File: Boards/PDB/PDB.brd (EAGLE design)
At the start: 160 x 101.6 mm, 49 parts, among them Q1 NMOS, Q2 IRFML8244, Q3 PMOS, Q4 PMOS, Q5 PMOS

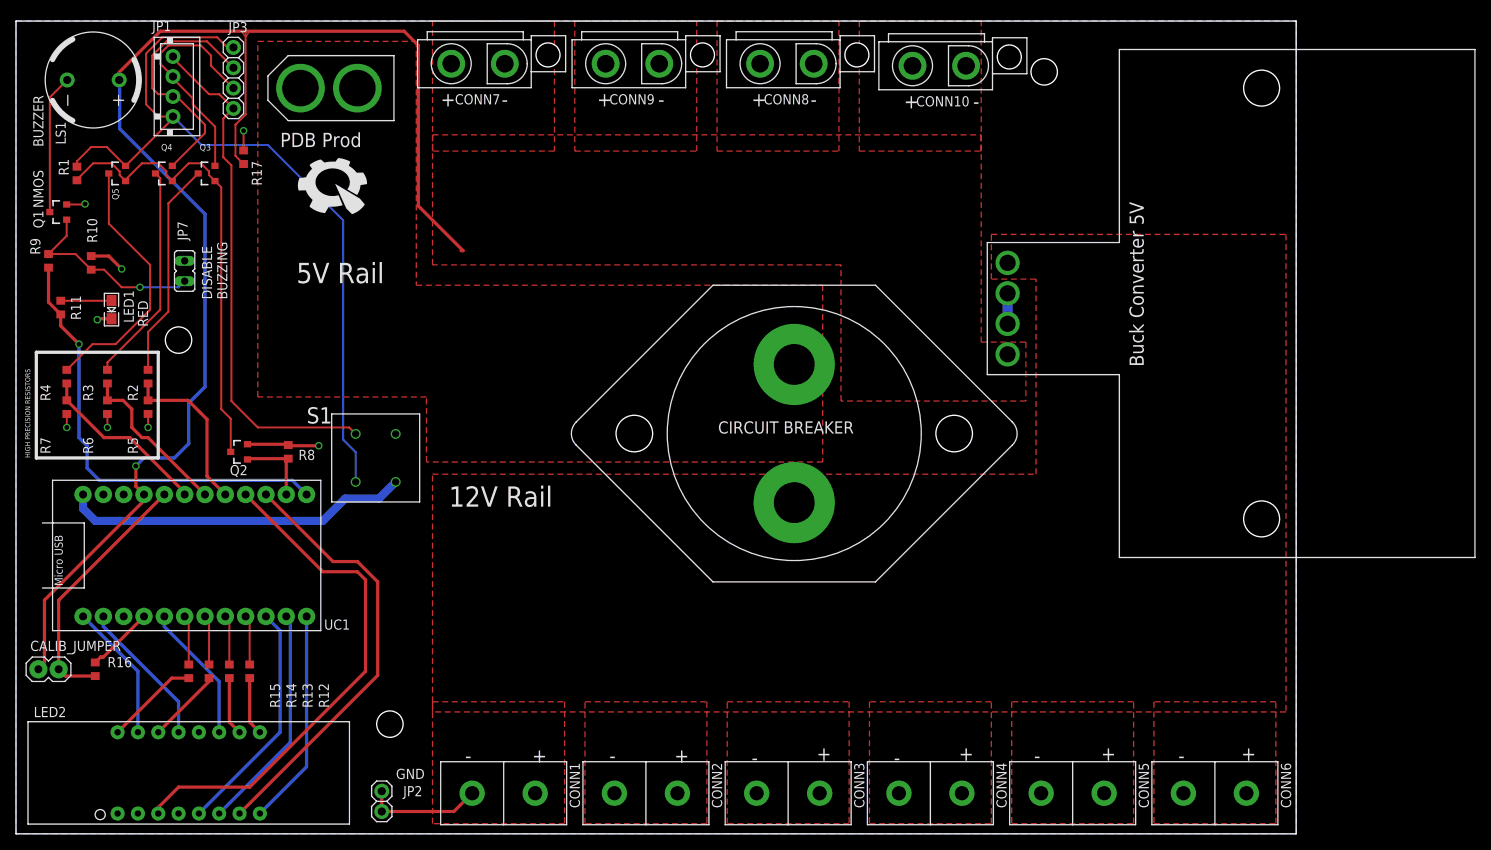
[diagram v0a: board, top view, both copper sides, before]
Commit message: REV B PLEASE WORK
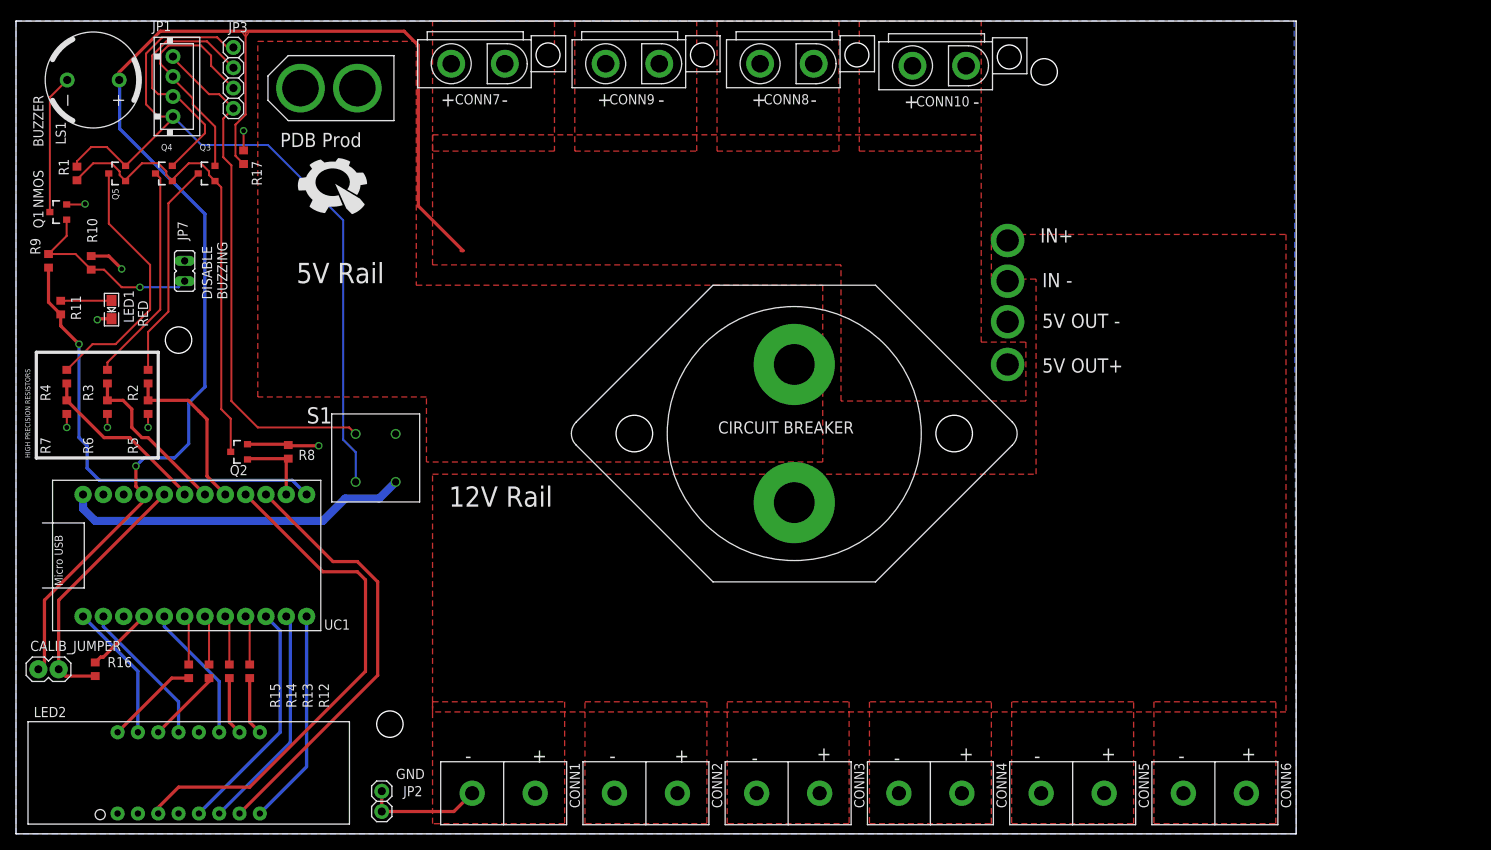
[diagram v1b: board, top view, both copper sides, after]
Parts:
- removed U$7: BUCK_CONVERTER_5V, pie:BUCK_CONVERTER_5V
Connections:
- net 12V: no longer U$7.IN+
- net 5V: no longer U$7.OUT+
- net GND: no longer U$7.IN-, U$7.OUT-
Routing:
- net GND: track 52.3 -> 48.5 mm, vias 8 -> 10
- net 5V: vias 1 -> 2
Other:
- board text added: "5V OUT -"
- board text added: "5V OUT+"
- board text added: "IN -"
- board text added: "IN+"
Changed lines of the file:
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@@
 <text x="80.264" y="90.932" size="1.778" layer="21">-</text>
 <text x="60.706" y="90.932" size="1.778" layer="21">-</text>
+<text x="128.016" y="73.914" size="1.778" layer="21">IN+</text>
+<text x="128.27" y="68.326" size="1.778" layer="21" font="vector">IN -</text>
+<text x="128.27" y="63.246" size="1.778" layer="21">5V OUT -</text>
+<text x="128.27" y="57.658" size="1.778" layer="21">5V OUT+</text>
 </plain>
 <attributes>
@@
 <element name="U$5" library="pie" package="STAND-OFF" value="" x="20.32" y="61.722"/>
 <element name="U$6" library="pie" package="PIE-LOGO-SMALL" value="" x="39.878" y="81.28"/>
-<element name="U$7" library="pie" package="BUCK_CONVERTER_5V" value="BUCK_CONVERTER_5V" x="155.702" y="66.294" smashed="yes" rot="R90"/>
 <element name="JP1" library="pie" package="XH_CONNECTOR_4POS_2.5MM" value="XH_CONN" x="19.812" y="93.218" smashed="yes" rot="R270">
 <attribute name="PIE-INT-REF-NUM" value="XH-4POS" x="71.882" y="104.648" size="1.778" layer="27" rot="R270" display="off"/>
@@
 <polygon width="1.1938" layer="16" rank="6">
 <vertex x="0" y="101.6"/>
-<vertex x="160.02" y="101.6"/>
+<vertex x="159.766" y="101.6"/>
 <vertex x="160.02" y="0"/>
 <vertex x="0" y="0"/>
@@
 <contactref element="CONN5" pad="PIN1"/>
 <contactref element="CONN6" pad="PIN1"/>
-<contactref element="U$7" pad="IN-"/>
-<contactref element="U$7" pad="OUT-"/>
 <contactref element="R5" pad="1"/>
 <contactref element="R6" pad="1"/>
@@
 <wire x1="10.922" y1="22.098" x2="10.58" y2="22.098" width="0.4064" layer="1"/>
 <wire x1="10.58" y1="22.098" x2="9.906" y2="21.424" width="0.4064" layer="1"/>
-<wire x1="123.952" y1="63.754" x2="123.952" y2="67.564" width="1.27" layer="16"/>
 <contactref element="CONN7" pad="P$2"/>
 <contactref element="CONN8" pad="P$2"/>
 <contactref element="CONN9" pad="P$2"/>
 <contactref element="CONN10" pad="P$2"/>
+<via x="123.952" y="69.088" extent="1-16" drill="2.8" diameter="3.81"/>
+<via x="123.952" y="64.008" extent="1-16" drill="2.8" diameter="3.81"/>
 </signal>
 <signal name="12V">
@@
 </polygon>
 <contactref element="CIRCUIT_BREAKER" pad="P$2"/>
-<contactref element="U$7" pad="IN+"/>
 <contactref element="CONN1" pad="PIN2"/>
 <polygon width="1.1938" layer="1" isolate="1.27">
@@
 <vertex x="142.24" y="16.51"/>
 </polygon>
+<via x="123.952" y="74.168" extent="1-16" drill="2.8" diameter="3.81"/>
 </signal>
 <signal name="BAT">
@@
 </signal>
 <signal name="5V">
-<contactref element="U$7" pad="OUT+"/>
 <polygon width="1.1938" layer="1">
 <vertex x="52.07" y="87.376"/>
@@
 </polygon>
 <contactref element="CONN10" pad="P$1"/>
+<via x="123.952" y="58.674" extent="1-16" drill="2.8" diameter="3.81"/>
 </signal>
 <signal name="IO1">
